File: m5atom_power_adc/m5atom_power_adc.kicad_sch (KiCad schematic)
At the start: 126 parts, among them J1 Conn_01x04_Socket, J10 Relay2, J11 R0SW, J12 R1SW, J13 R2SW, J14 Conn_01x02, J2 GROVE-CONNECTOR, J3 Conn_01x04_Pin, J4 USB_C_Receptacle_USB2.0_16P, J5 SubBatt, J6 MainBatt, J7 Relay0, J8 Relay1, J9 GROVE-CONNECTOR, Q1 AO3401A, Q2 MMBT2222A, Q3 MMBT2222A, Q4 MMBT2222A, Q5 AO3401A, Q6 MMBT2222A, Q7 MMBT2222A, Q8 AO3401A, Q9 MMBT2222A, SW1 Boot, SW2 Reset, U1 LM2596S-5, U2 ESP32-S3-MINI-1, U3 AMS1117-3.3, U4 ADS1115IDGS, U5 AMS1117-3.3, U6 LTC2944

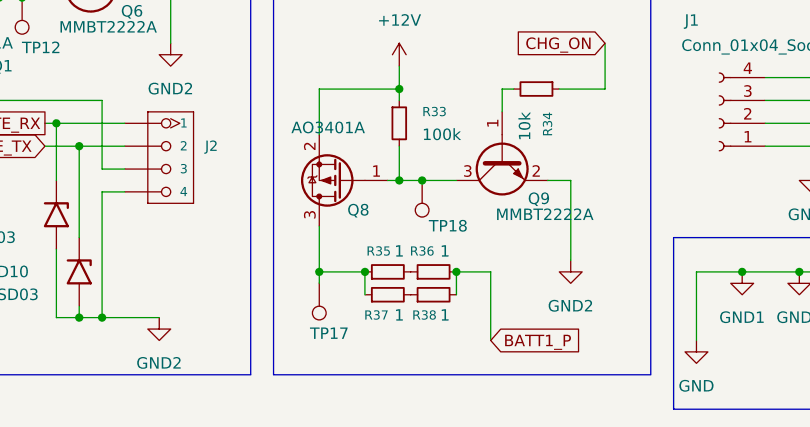
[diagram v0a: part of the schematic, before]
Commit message: fix: 部品選定を進めた。あとはSWだけ。
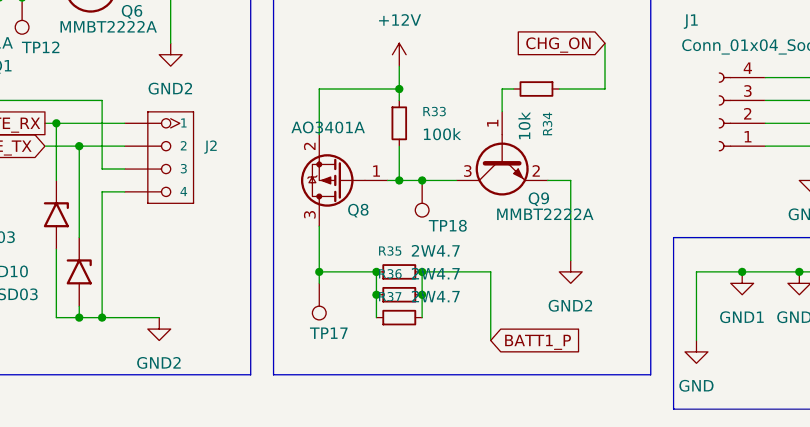
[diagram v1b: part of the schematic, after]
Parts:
- removed R38: 1, symbol Device:R_Small
- R1, R14, R15, R17, R22, R34, R6, R7: footprint (none) -> Resistor_SMD:R_0402_1005Metric; JLC_Num (none) -> C2906862
- R10, R11, R12, R13: footprint (none) -> Resistor_SMD:R_0402_1005Metric; JLC_Num (none) -> C705627
- R16, R19, R20, R25: footprint (none) -> Resistor_SMD:R_0603_1608Metric; JLC_Num (none) -> C21190
- R18, R21, R27, R29, R31, R33: footprint (none) -> Resistor_SMD:R_0603_1608Metric; JLC_Num (none) -> C2906981
- R2, R23, R24, R26, R3: footprint (none) -> Resistor_SMD:R_0603_1608Metric; JLC_Num (none) -> C2907045
- R28, R30, R32: footprint (none) -> Resistor_SMD:R_0603_1608Metric; JLC_Num (none) -> C22967
- R35, R36, R37: value 1 -> 2W4.7; footprint (none) -> Resistor_SMD:R_2512_6332Metric; JLC_Num (none) -> C876270
- R4, R8: footprint (none) -> Resistor_SMD:R_0603_1608Metric; JLC_Num (none) -> C2989042
- R5, R9: footprint (none) -> Resistor_SMD:R_0402_1005Metric; JLC_Num (none) -> C326601
- U6: footprint (none) -> Package_DFN_QFN:DFN-8-1EP_3x3mm_P0.5mm_EP1.65x2.38mm; JLC_Num (none) -> C683672
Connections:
- net BATT1_P: now also R35.2, R37.2
- net at R36.1: now also Q8.3 (D), R35.1, R37.1, TP17.1; no longer R35.2
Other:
- moved on the sheet: R35
